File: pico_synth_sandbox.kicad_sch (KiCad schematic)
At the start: 22 parts, among them J1 Micro_SD_Card_Det2, SW1 RotaryEncoder_Switch, SW2 RotaryEncoder_Switch, SW3 PWR_EN, U1 Pico, U2 MIC5219-3.3YM5

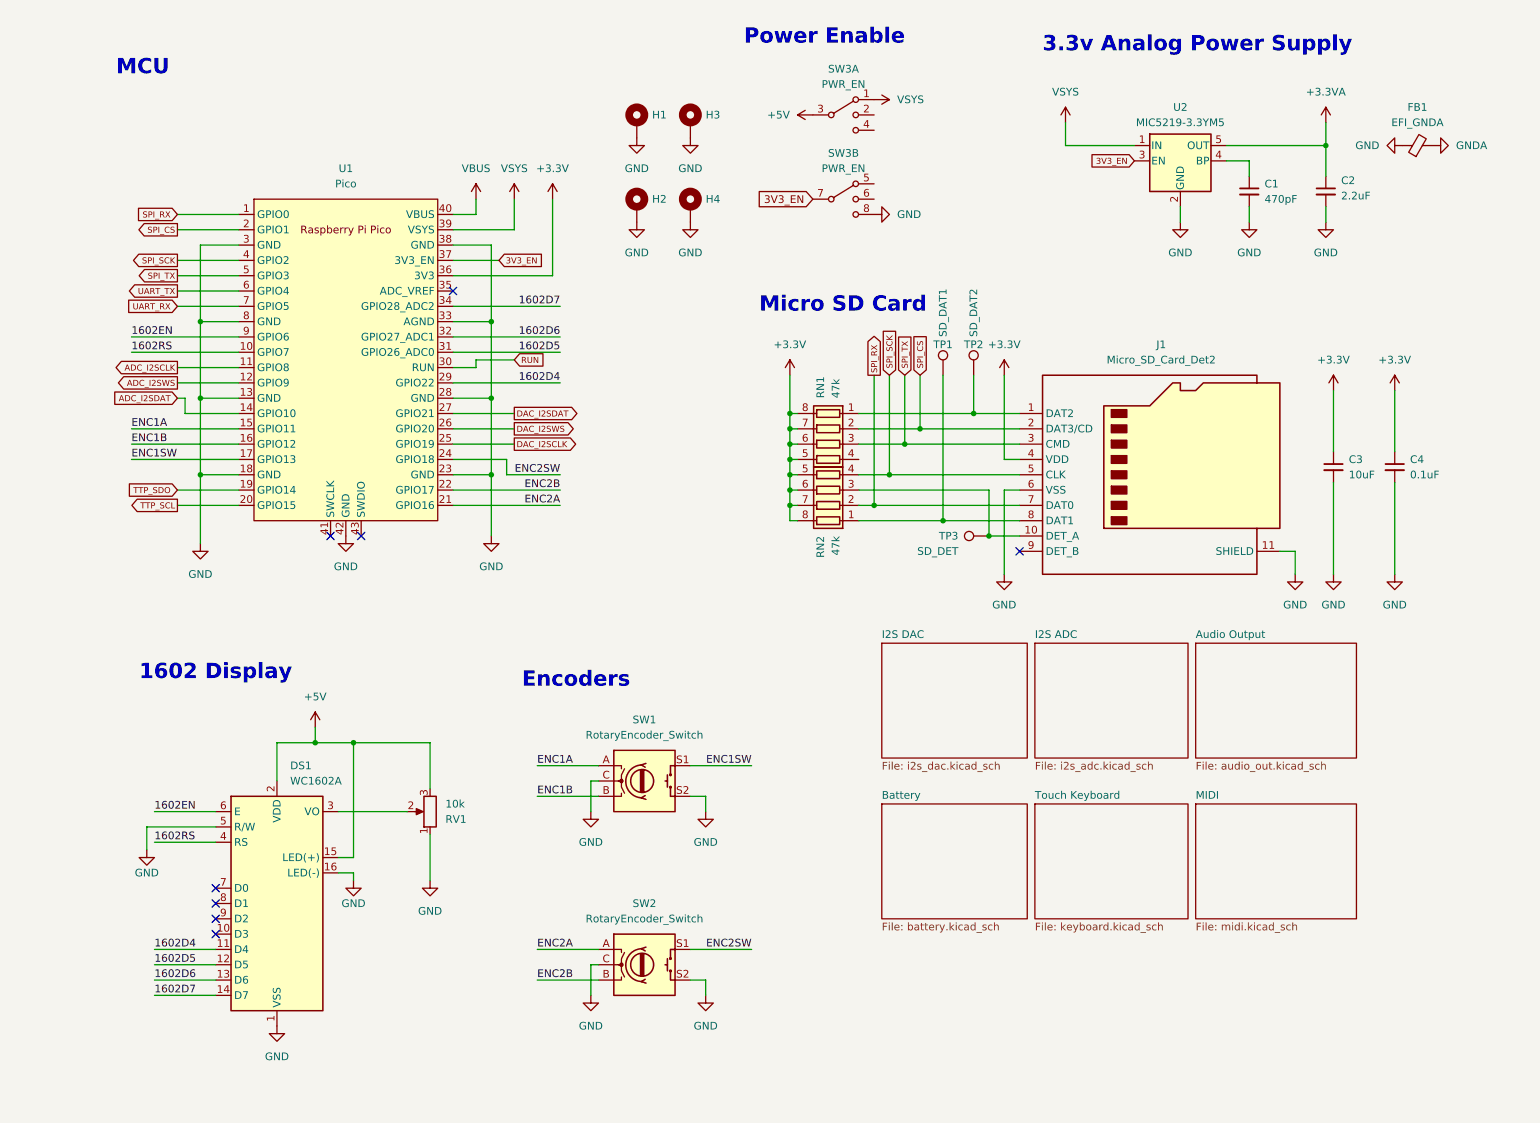
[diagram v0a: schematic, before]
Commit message: Initial schematic of Rev3.
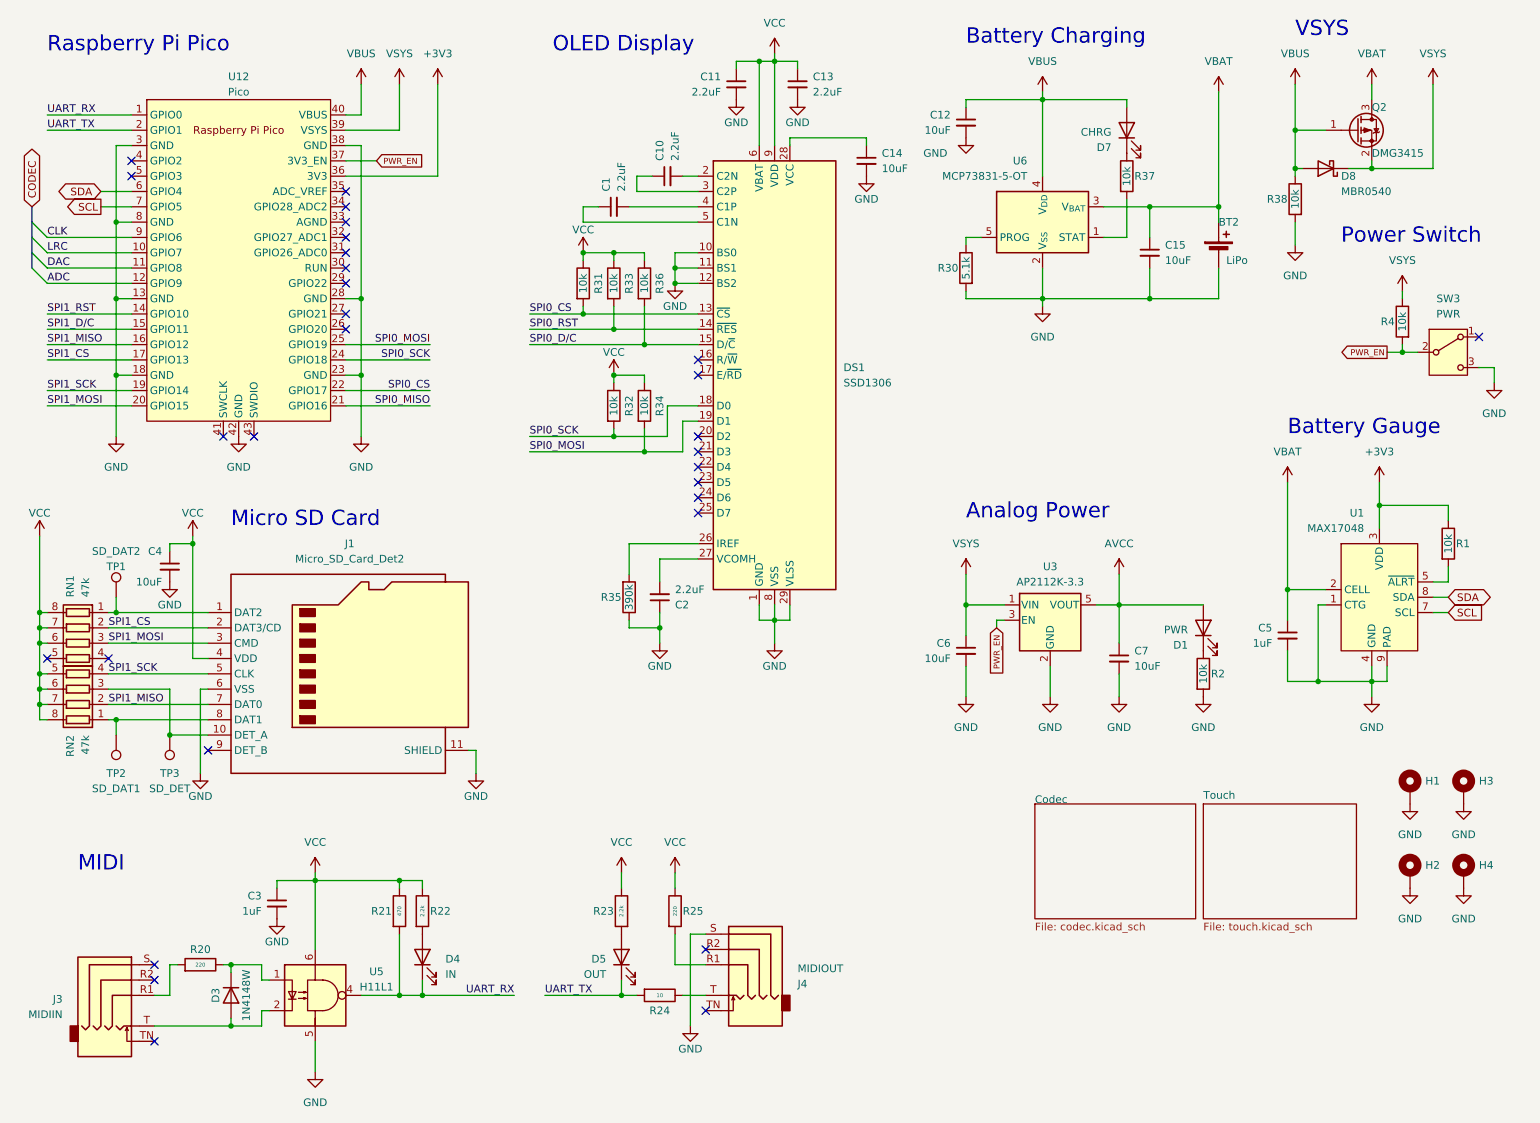
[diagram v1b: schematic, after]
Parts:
- removed DS1: WC1602A, Display:WC1602A, symbol Display_Character:WC1602A
- removed FB1: EFI_GNDA, Resistor_SMD:R_0805_2012Metric_Pad1.20x1.40mm_HandSolder, symbol Device:FerriteBead_Small
- removed RV1: 10k, Potentiometer_THT:Potentiometer_Runtron_RM-065_Vertical, symbol Device:R_Potentiometer
- removed SW1, SW2: RotaryEncoder_Switch, Rotary_Encoder:RotaryEncoder_Alps_EC11E-Switch_Vertical_H20mm, symbol Device:RotaryEncoder_Switch
- removed SW3: PWR_EN, pico_synth_sandbox:MK-23D38, symbol Switch:SW_DP3T
- removed U1: Pico, pico_synth_sandbox:RPi_Pico_SMD_TH_BS, symbol MCU_RaspberryPi_and_Boards:Pico
- removed U2: MIC5219-3.3YM5, Package_TO_SOT_SMD:SOT-23-5, symbol Regulator_Linear:MIC5219-3.3YM5
- added BT2: LiPo, Connector_JST:JST_PH_S2B-PH-SM4-TB_1x02-1MP_P2.00mm_Horizontal, symbol Device:Battery_Cell
- added C10, C11, C13: 2.2uF, symbol Device:C_Small
- added C12, C15, C6, C7: 10uF, Capacitor_SMD:C_0805_2012Metric_Pad1.18x1.45mm_HandSolder, symbol Device:C_Small
- added C14: 10uF, symbol Device:C_Small
- added C5: 1uF, Capacitor_SMD:C_0805_2012Metric_Pad1.18x1.45mm_HandSolder, symbol Device:C_Small
- added D1: PWR, LED_SMD:LED_0805_2012Metric_Pad1.15x1.40mm_HandSolder, symbol Device:LED
- added D3: 1N4148W, Diode_SMD:D_SOD-123, symbol Diode:1N4148W
- added D4: IN, LED_SMD:LED_0805_2012Metric_Pad1.15x1.40mm_HandSolder, symbol Device:LED
- added D5: OUT, LED_SMD:LED_0805_2012Metric_Pad1.15x1.40mm_HandSolder, symbol Device:LED
- added D7: CHRG, LED_SMD:LED_0805_2012Metric_Pad1.15x1.40mm_HandSolder, symbol Device:LED
- added D8: MBR0540, Diode_SMD:D_SOD-123, symbol Diode:MBR0540
- added DS1: SSD1306, Display:OLED-128O064D, symbol Display_Graphic:OLED-128O064D
- added J3: MIDIIN, pico_synth_sandbox:Jack_3.5mm_PJ327A_Horizontal, symbol Connector_Audio:AudioJack4_SwitchT1
- added J4: MIDIOUT, pico_synth_sandbox:Jack_3.5mm_PJ327A_Horizontal, symbol Connector_Audio:AudioJack4_SwitchT1
- added Q2: DMG3415, Package_TO_SOT_SMD:SOT-23_Handsoldering, symbol Transistor_FET:BSS84
- added R1, R2, R37, R38, R4: 10k, Resistor_SMD:R_0805_2012Metric_Pad1.20x1.40mm_HandSolder, symbol Device:R
- added R20, R25: 220, Resistor_SMD:R_0805_2012Metric_Pad1.20x1.40mm_HandSolder, symbol Device:R
- added R21: 470, Resistor_SMD:R_0805_2012Metric_Pad1.20x1.40mm_HandSolder, symbol Device:R
- added R22, R23: 2.2k, Resistor_SMD:R_0805_2012Metric_Pad1.20x1.40mm_HandSolder, symbol Device:R
- added R24: 10, Resistor_SMD:R_0805_2012Metric_Pad1.20x1.40mm_HandSolder, symbol Device:R
- added R30: 5.1k, Resistor_SMD:R_0805_2012Metric_Pad1.20x1.40mm_HandSolder, symbol Device:R
- added R31, R32, R33, R34, R36: 10k, symbol Device:R
- added R35: 390k, symbol Device:R
- added SW3: PWR, symbol Switch:SW_SPDT
- added U1: MAX17048, Package_DFN_QFN:TDFN-8-1EP_2x2mm_P0.5mm_EP0.8x1.2mm, symbol pico_synth_sandbox:MAX17048
- added U12: Pico, RPi_Pico:RPi_Pico_SMD_TH, symbol MCU_RaspberryPi_and_Boards:Pico
- added U3: AP2112K-3.3, Package_TO_SOT_SMD:SOT-23-5, symbol Regulator_Linear:AP2112K-3.3
- added U5: H11L1, Package_DIP:SMDIP-6_W7.62mm, symbol Isolator:H11L1
- added U6: MCP73831-5-OT, Package_TO_SOT_SMD:SOT-23-5, symbol Battery_Management:MCP73831-5-OT
- C1: value 470pF -> 2.2uF; footprint Capacitor_SMD:C_0805_2012Metric_Pad1.18x1.45mm_HandSolder -> (none)
- C2: footprint Capacitor_SMD:C_0805_2012Metric_Pad1.18x1.45mm_HandSolder -> (none)
- C3: value 10uF -> 1uF
- C4: value 0.1uF -> 10uF
- TP1: value SD_DAT1 -> SD_DAT2
- TP2: value SD_DAT2 -> SD_DAT1
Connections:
- net +3.3VA is gone; now on net GND: C2.1
- net GND: now also BT2.2 (-), C11.2, C12.2, C13.2, C14.2, C15.2, C5.2, C6.2, C7.2, DS1.1 (GND), DS1.10 (BS0), DS1.11 (BS1), DS1.12 (BS2), DS1.29 (VLSS), DS1.30 (GND), DS1.8 (VSS), J4.S, R2.2, R30.2, R35.1, R38.2, SW3.3 (C), U1.1 (CTG), U1.4 (GND), U1.9 (PAD), U12.13 (GND), U12.18 (GND), U12.23 (GND), U12.28 (GND), U12.3 (GND), U12.38 (GND), U12.42 (GND), U12.8 (GND), U3.2 (GND), U5.5, U6.2 (V_{SS}); no longer C1.2, C2.2
- net UART_RX: now also D4.1 (K), R21.2, U12.1 (GPIO0), U5.4
- net UART_TX: now also D5.1 (K), R24.2, U12.2 (GPIO1)
- net VBUS: now also C12.1, D7.2 (A), D8.2 (A), Q2.1 (G), R38.1, U12.40 (VBUS), U6.4 (V_{DD})
- net VSYS: now also C6.1, D8.1 (K), Q2.2 (S), R4.1, U12.39 (VSYS), U3.1 (VIN)
- net at J1.1 (DAT2), RN1.1 (R1.1): now also TP1.1; no longer TP2.1
- net at J1.8 (DAT1), RN2.1 (R1.1): now also TP2.1; no longer TP1.1
- net at C1.1: now also DS1.5 (C1N)
- net +3.3V renamed VCC
- net VCC: now also C11.1, C13.1, DS1.6 (VBAT), DS1.9 (VDD), R21.1, R22.1, R23.1, R25.1, R31.1, R32.1, R33.1, R34.1, R36.1, U5.6; no longer RN1.5 (R4.2)
- net SPI_CS renamed SPI1_CS
- net SPI1_CS: now also U12.17 (GPIO13)
- net SPI_RX renamed SPI1_MISO
- net SPI1_MISO: now also U12.16 (GPIO12)
- net SPI_SCK renamed SPI1_SCK
- net SPI1_SCK: now also U12.19 (GPIO14)
- net SPI_TX renamed SPI1_MOSI
- net SPI1_MOSI: now also U12.20 (GPIO15)
- new net: C14.1, DS1.28 (VCC)
- new net: D3.1 (K), R20.1, U5.1
- new net: J3.R1, R20.2
- new net: R1.2, U1.5 (~{ALRT})
- new net: C10.1, DS1.3 (C2P)
- new net: C10.2, DS1.2 (C2N)
- new net: R37.2, U6.1 (STAT)
- new net: R30.1, U6.5 (PROG)
- new net: D7.1 (K), R37.1
- new net: J4.R1, R25.2
- new net: D5.2 (A), R23.2
- new net: D1.1 (K), R2.1
- new net: D3.2 (A), J3.T, U5.2
- new net: J4.T, R24.1
- new net: DS1.26 (IREF), R35.2
- new net: C2.2, DS1.27 (VCOMH)
- new net: C1.2, DS1.4 (C1P)
- new net: D4.2 (A), R22.2
- new net +3V3: R1.1, U1.3 (VDD), U12.36 (3V3)
- new net ADC: U12.12 (GPIO9)
- new net AVCC: C7.1, D1.2 (A), U3.5 (VOUT)
- new net CLK: U12.9 (GPIO6)
- new net DAC: U12.11 (GPIO8)
- new net LRC: U12.10 (GPIO7)
- new net PWR_EN: R4.2, SW3.2 (B), U12.37 (3V3_EN), U3.3 (EN)
- new net SCL: U1.7 (SCL), U12.7 (GPIO5)
- new net SDA: U1.8 (SDA), U12.6 (GPIO4)
- new net SPI0_CS: DS1.13 (~{CS}), R31.2, U12.22 (GPIO17)
- new net SPI0_D/C: DS1.15 (D/~{C}), R36.2
- new net SPI0_MISO: U12.21 (GPIO16)
- new net SPI0_MOSI: DS1.19 (D1), R34.2, U12.25 (GPIO19)
- new net SPI0_RST: DS1.14 (~{RES}), R33.2
- new net SPI0_SCK: DS1.18 (D0), R32.2, U12.24 (GPIO18)
- new net SPI1_D/C: U12.15 (GPIO11)
- new net SPI1_RST: U12.14 (GPIO10)
- new net VBAT: BT2.1 (+), C15.1, C5.1, Q2.3 (D), U1.2 (CELL), U6.3 (V_{BAT})
- no-connect marks 8 -> 30
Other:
- sheet Audio Output renamed Codec
- sheet Touch Keyboard renamed Touch
- removed sheet Battery
- removed sheet I2S ADC
- removed sheet I2S DAC
- removed sheet MIDI
- sheet Codec: file audio_out.kicad_sch -> codec.kicad_sch
- sheet Touch: file keyboard.kicad_sch -> touch.kicad_sch
- note added: "Analog Power"
- note added: "Battery Charging"
- note added: "Battery Gauge"
- note added: "MIDI"
- note added: "OLED Display"
- note added: "Power Switch"
- note added: "Raspberry Pi Pico"
- note added: "VSYS"
- note removed: "1602 Display"
- note removed: "3.3v Analog Power Supply"
- note removed: "Encoders"
- note removed: "MCU"
- note removed: "Power Enable"
- moved on the sheet: H1, H2, H3, H4
